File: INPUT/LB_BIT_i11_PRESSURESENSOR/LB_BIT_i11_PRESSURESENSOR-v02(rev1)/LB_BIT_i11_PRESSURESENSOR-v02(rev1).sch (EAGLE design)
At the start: 11 parts

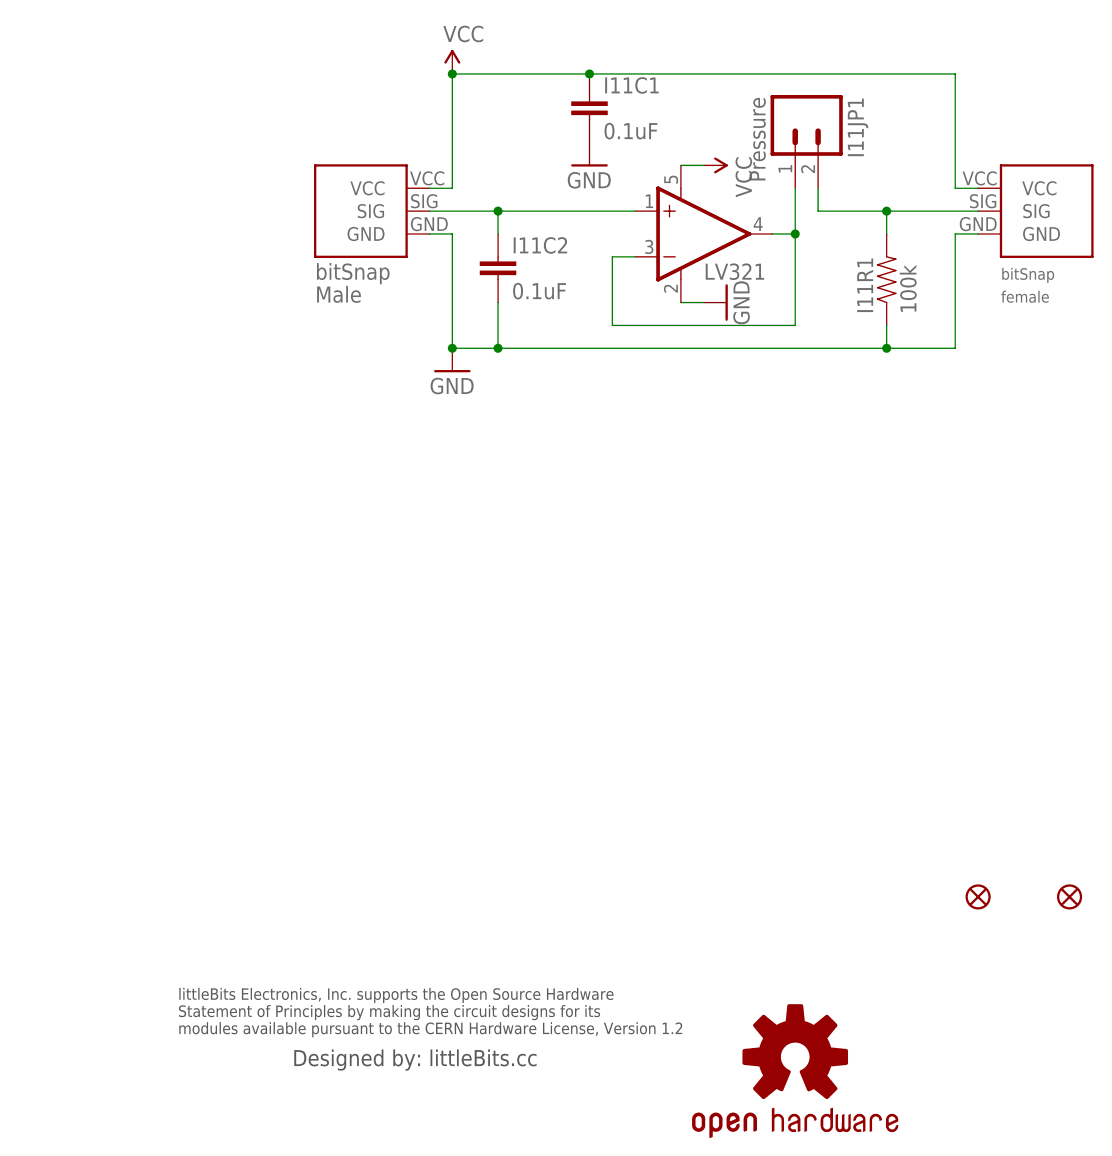
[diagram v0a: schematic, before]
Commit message: Updated license text
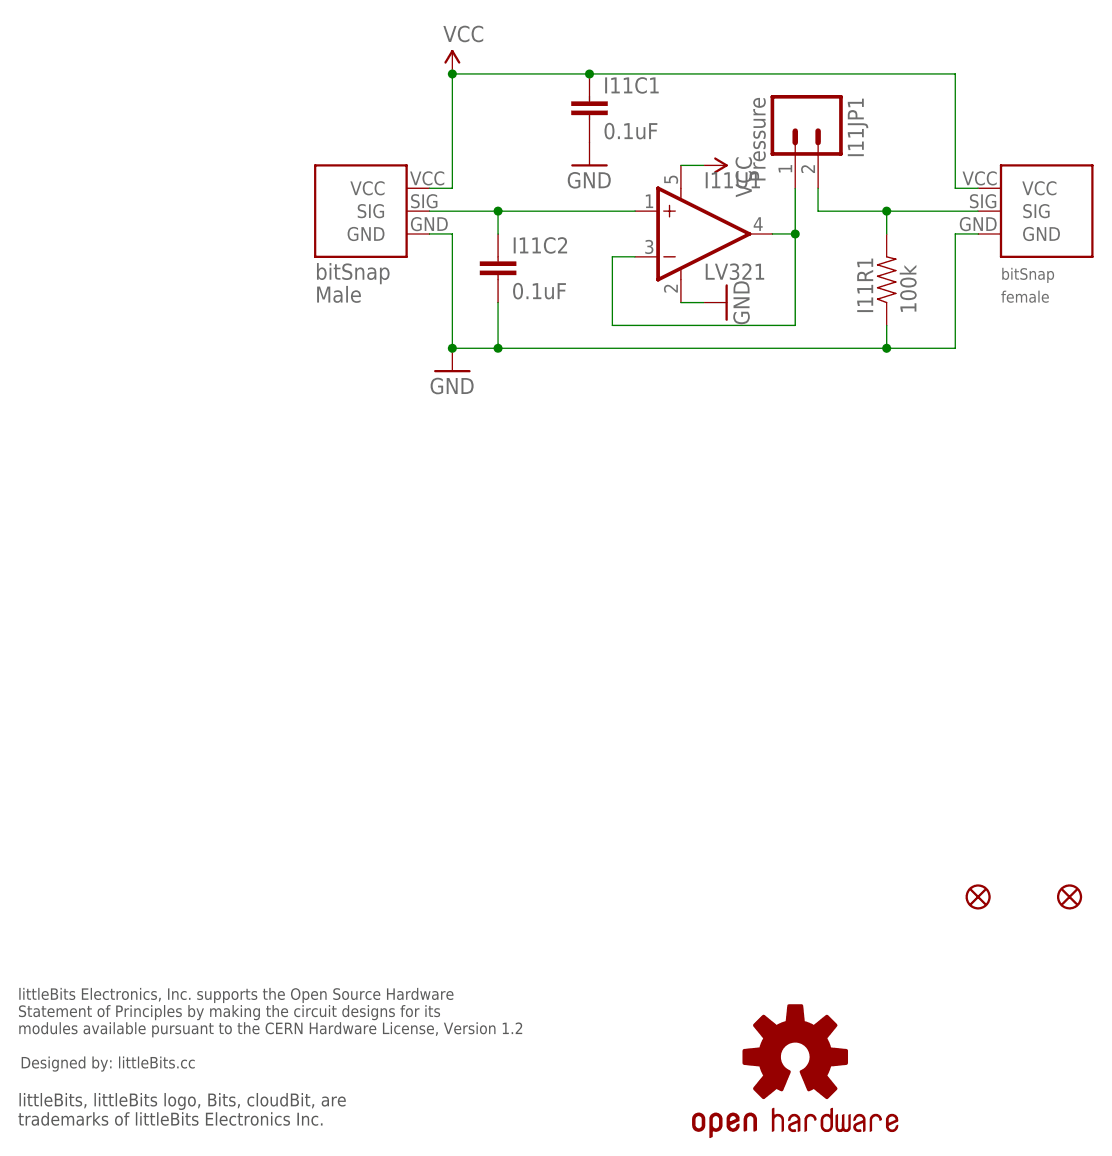
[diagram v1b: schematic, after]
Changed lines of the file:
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@@
 <instance part="GND3" gate="1" x="109.22" y="109.22"/>
 <instance part="I11U1" gate="G$1" x="121.92" y="101.6"/>
-<instance part="U$1" gate="G$1" x="63.5" y="7.62"/>
+<instance part="U$1" gate="G$1" x="45.72" y="7.62"/>
 </instances>
 <busses>
